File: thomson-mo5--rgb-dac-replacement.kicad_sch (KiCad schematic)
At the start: 2 parts, among them J101 Input, J102 Output

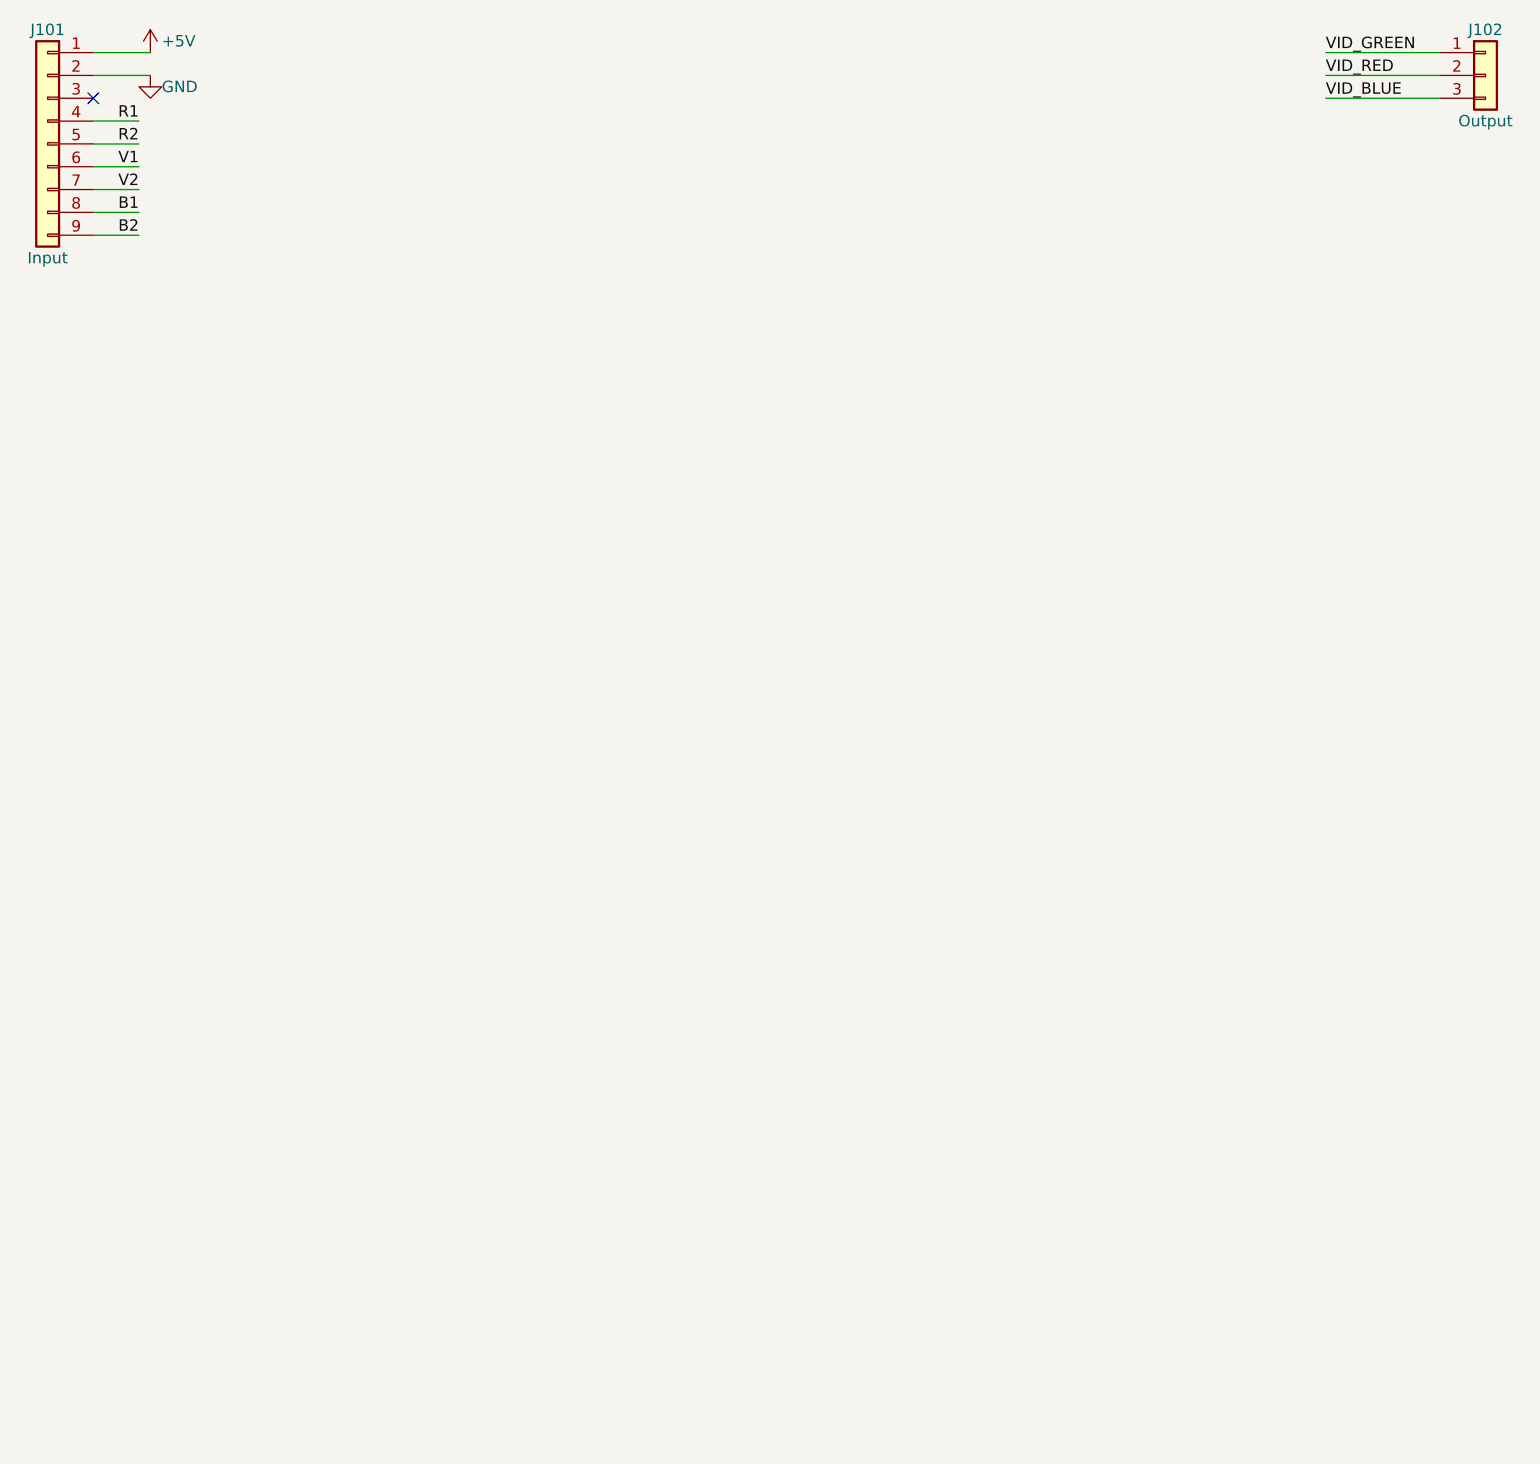
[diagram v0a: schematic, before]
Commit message: Done schematis
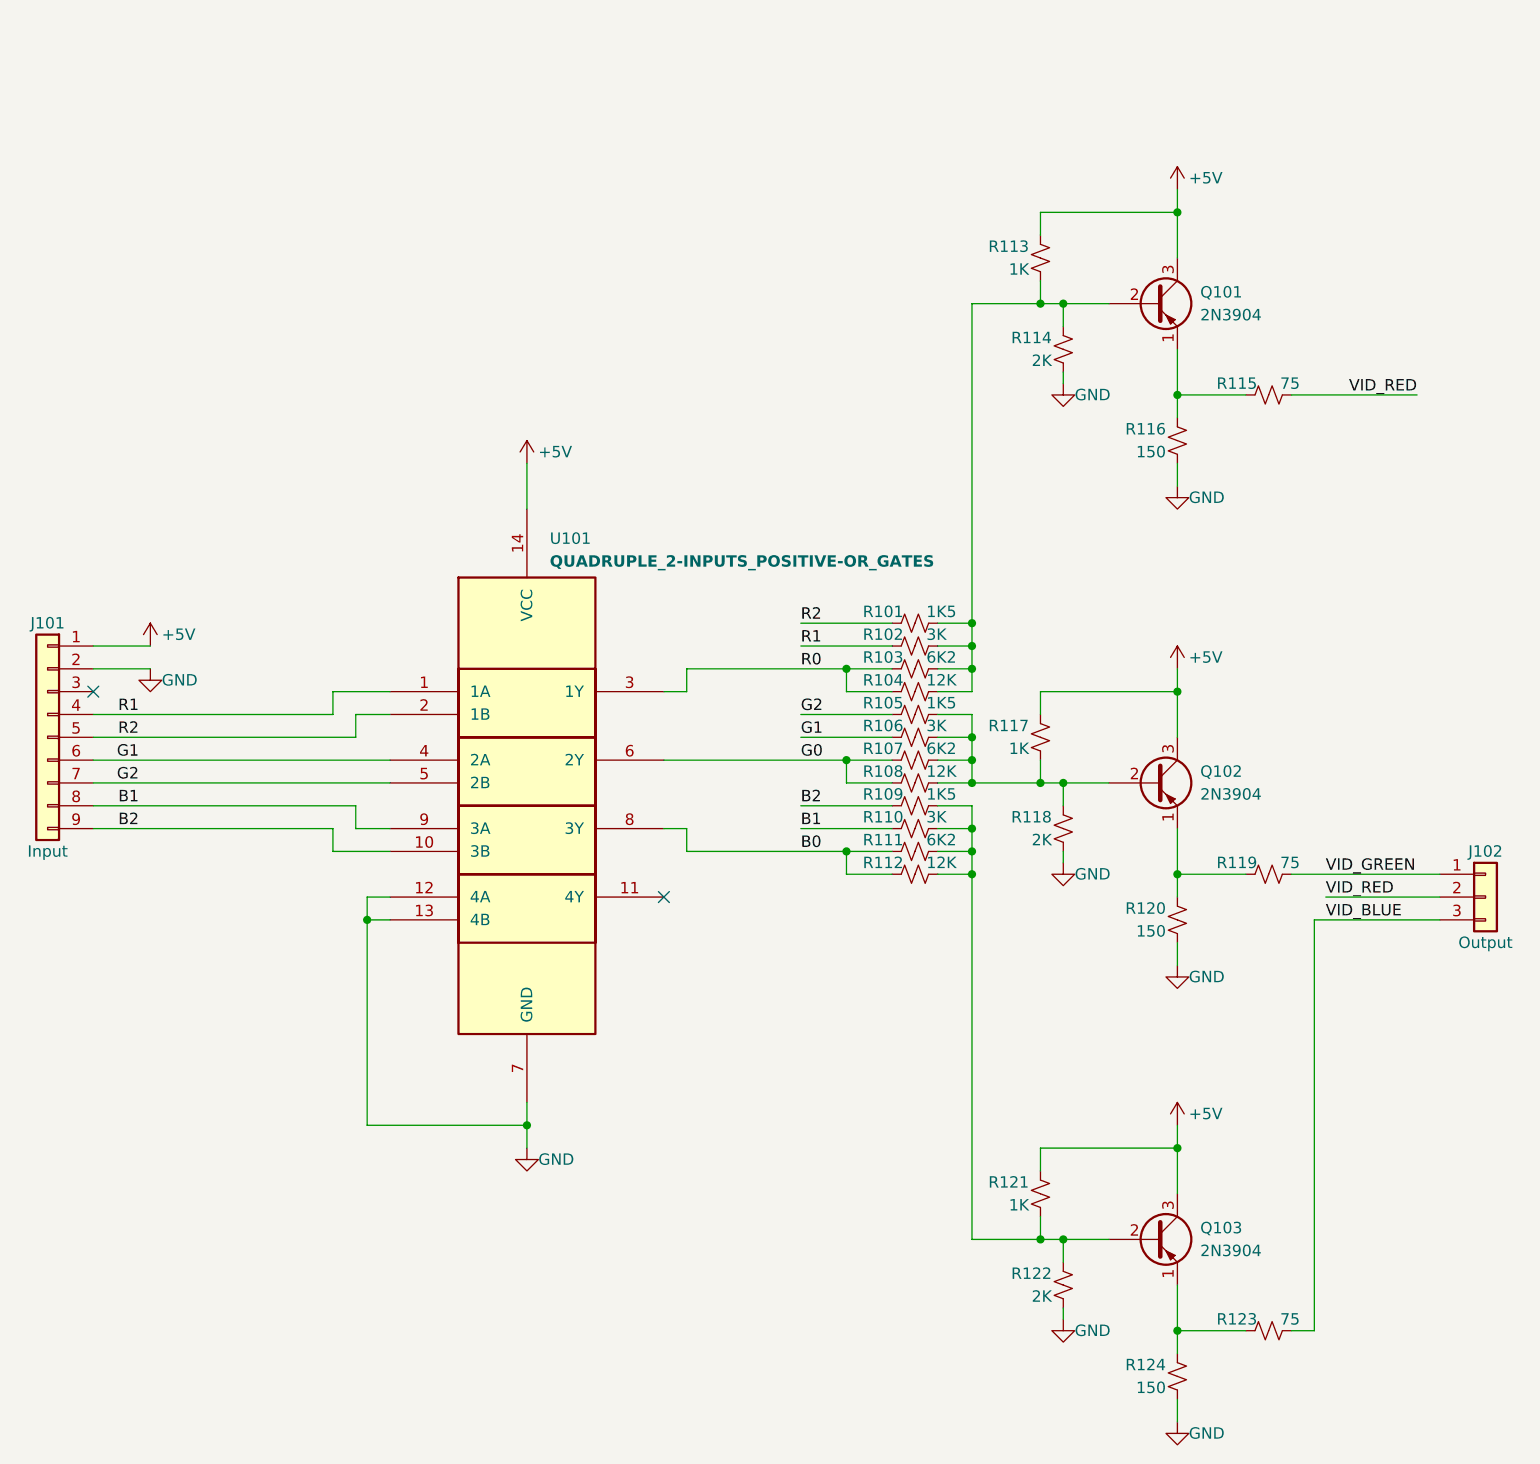
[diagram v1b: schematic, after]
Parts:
- added Q101, Q102, Q103: 2N3904, symbol Device:Q_PNP_EBC
- added R101, R105, R109: 1K5, symbol Device:R_Small_US
- added R102, R106, R110: 3K, symbol Device:R_Small_US
- added R103, R107, R111: 6K2, symbol Device:R_Small_US
- added R104, R108, R112: 12K, symbol Device:R_Small_US
- added R113, R117, R121: 1K, symbol Device:R_Small_US
- added R114, R118, R122: 2K, symbol Device:R_Small_US
- added R115, R119, R123: 75, symbol Device:R_Small_US
- added R116, R120, R124: 150, symbol Device:R_Small_US
- added U101: QUADRUPLE_2-INPUTS_POSITIVE-OR_GATES, Package_DIP:DIP-14_W7.62mm_LongPads, symbol 74x32:QUADRUPLE_2-INPUTS_POSITIVE-OR_GATES
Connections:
- net +5V: now also Q101.3 (C), Q102.3 (C), Q103.3 (C), R113.2, R117.2, R121.2, U101.14 (VCC)
- net B1: now also R110.1, U101.9 (3A)
- net B2: now also R109.1, U101.10 (3B)
- net GND: now also R114.1, R116.1, R118.1, R120.1, R122.1, R124.1, U101.12 (4A), U101.13 (4B), U101.7 (GND)
- net R1: now also R102.1, U101.1 (1A)
- net R2: now also R101.1, U101.2 (1B)
- net VID_BLUE: now also R123.2
- net VID_GREEN: now also R119.2
- net VID_RED: now also R115.2
- net V1 renamed G1
- net G1: now also R106.1, U101.4 (2A)
- net V2 renamed G2
- net G2: now also R105.1, U101.5 (2B)
- new net: Q101.1 (E), R115.1, R116.2
- new net: Q101.2 (B), R101.2, R102.2, R103.2, R104.2, R113.1, R114.2
- new net: Q102.1 (E), R119.1, R120.2
- new net: Q102.2 (B), R105.2, R106.2, R107.2, R108.2, R117.1, R118.2
- new net: Q103.1 (E), R123.1, R124.2
- new net: Q103.2 (B), R109.2, R110.2, R111.2, R112.2, R121.1, R122.2
- new net B0: R111.1, R112.1, U101.8 (3Y)
- new net G0: R107.1, R108.1, U101.6 (2Y)
- new net R0: R103.1, R104.1, U101.3 (1Y)
- no-connect marks 1 -> 2
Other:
- moved on the sheet: J101, J102
